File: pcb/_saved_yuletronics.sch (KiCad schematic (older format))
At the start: 52 parts, among them IC1 STM32F042F6P6, IC3 TLV61225, J1 BATT, J2 MICROUSB, J3 CONN_01x08, P1 SWD_TC, SW1 BOOTLOAD, SW2 PWR_SWITCH, SW3 BOOTLOAD, U1 XC6210B332MR, U2 ULN2003D1013TR, X1 Silk_art

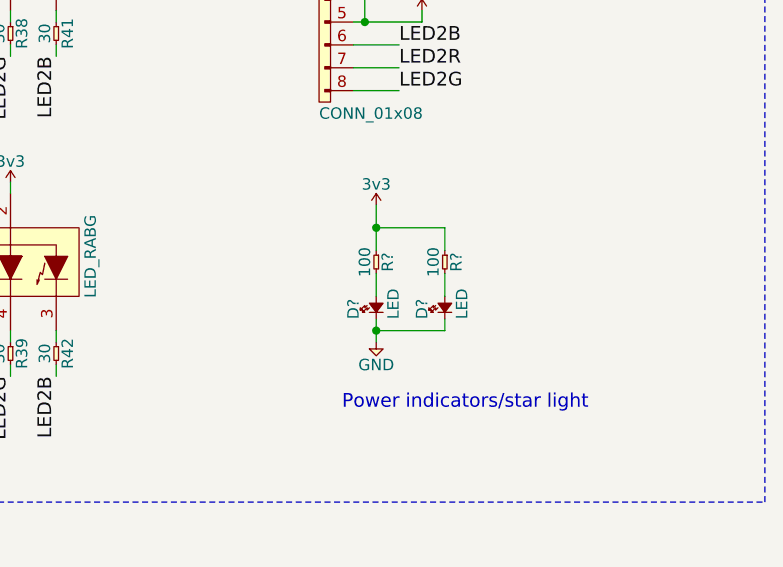
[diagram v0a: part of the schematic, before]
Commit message: Fix circuit to account for LED currents: change resistor values, upgrade LDO regulator, use transistor array
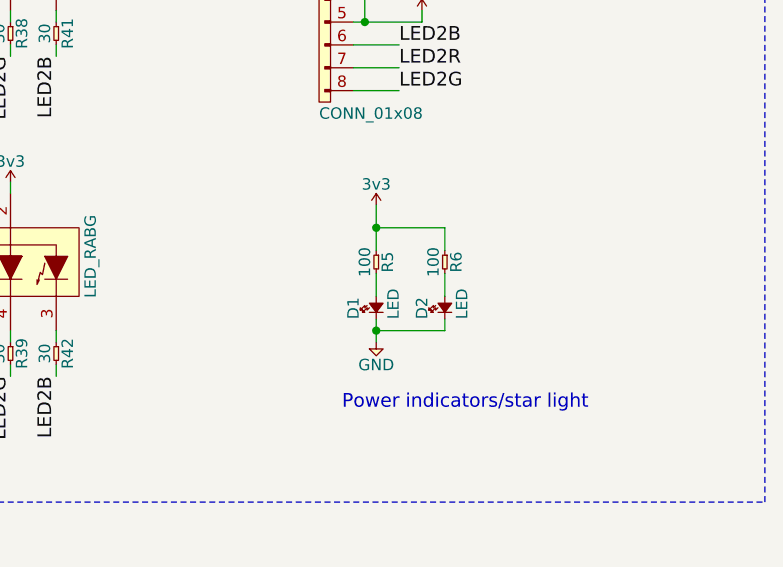
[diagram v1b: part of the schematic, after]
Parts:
- gave numbers to parts that had none: 4
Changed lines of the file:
@@
 	4250 5350 4250 5200
 $Comp
-L LED D?
+L LED D1
 U 1 1 58097B31
 P 9200 4700
-F 0 "D?" H 9200 4800 50  0000 L CNN
+F 0 "D1" H 9200 4800 50  0000 L CNN
 F 1 "LED" H 9200 4625 50  0000 L CNN
 F 2 "agg:0805-LED" H 9200 4700 50  0001 C CNN
@@
 $EndComp
 $Comp
-L 3v3 #PWR?
+L 3v3 #PWR038
 U 1 1 58098160
 P 9200 4200
-F 0 "#PWR?" H 9200 4310 50  0001 L CNN
+F 0 "#PWR038" H 9200 4310 50  0001 L CNN
 F 1 "3v3" H 9200 4290 50  0000 C CNN
 F 2 "" H 9200 4200 60  0001 C CNN
@@
 $EndComp
 $Comp
-L GND #PWR?
+L GND #PWR039
 U 1 1 580987D6
 P 9200 4800
-F 0 "#PWR?" H 9070 4840 50  0001 L CNN
+F 0 "#PWR039" H 9070 4840 50  0001 L CNN
 F 1 "GND" H 9200 4700 50  0000 C CNN
 F 2 "" H 9200 4800 60  0001 C CNN
@@
 Power indicators/star light
 $Comp
-L LED D?
+L LED D2
 U 1 1 580998C3
 P 9500 4700
-F 0 "D?" H 9500 4800 50  0000 L CNN
+F 0 "D2" H 9500 4800 50  0000 L CNN
 F 1 "LED" H 9500 4625 50  0000 L CNN
 F 2 "agg:0805-LED" H 9500 4700 50  0001 C CNN
@@
 $EndComp
 $Comp
-L R R?
+L R R5
 U 1 1 58099A5B
 P 9200 4400
-F 0 "R?" H 9250 4450 50  0000 C CNN
+F 0 "R5" H 9250 4450 50  0000 C CNN
 F 1 "100" H 9250 4350 50  0000 C CNN
 F 2 "agg:0805" H 9200 4400 50  0001 C CNN
@@
 $EndComp
 $Comp
-L R R?
+L R R6
 U 1 1 58099CFF
 P 9500 4400
-F 0 "R?" H 9550 4450 50  0000 C CNN
+F 0 "R6" H 9550 4450 50  0000 C CNN
 F 1 "100" H 9550 4350 50  0000 C CNN
 F 2 "agg:0805" H 9500 4400 50  0001 C CNN

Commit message: Further configuration, create initial board.h file
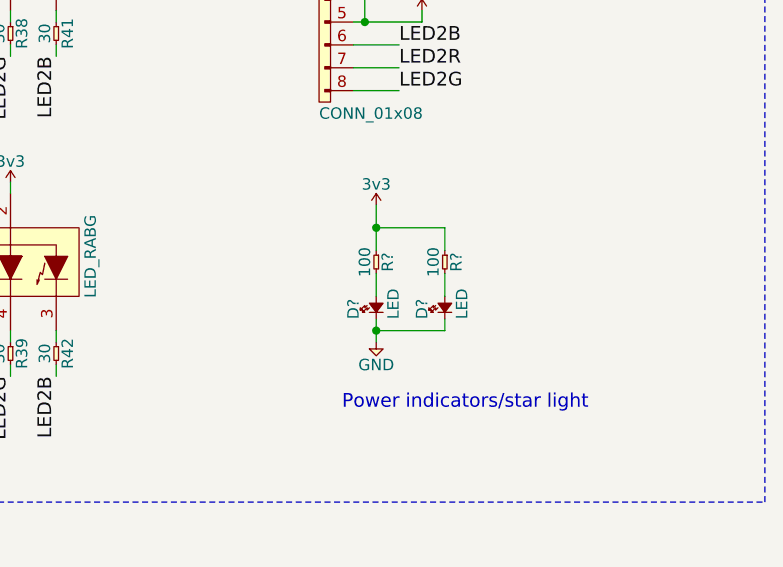
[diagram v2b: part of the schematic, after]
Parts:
- renumbered D1 to D?, D2 to D?, R5 to R?, R6 to R?
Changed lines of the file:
@@
 	4250 5350 4250 5200
 $Comp
-L LED D1
+L LED D?
 U 1 1 58097B31
 P 9200 4700
-F 0 "D1" H 9200 4800 50  0000 L CNN
+F 0 "D?" H 9200 4800 50  0000 L CNN
 F 1 "LED" H 9200 4625 50  0000 L CNN
 F 2 "agg:0805-LED" H 9200 4700 50  0001 C CNN
@@
 $EndComp
 $Comp
-L 3v3 #PWR038
+L 3v3 #PWR?
 U 1 1 58098160
 P 9200 4200
-F 0 "#PWR038" H 9200 4310 50  0001 L CNN
+F 0 "#PWR?" H 9200 4310 50  0001 L CNN
 F 1 "3v3" H 9200 4290 50  0000 C CNN
 F 2 "" H 9200 4200 60  0001 C CNN
@@
 $EndComp
 $Comp
-L GND #PWR039
+L GND #PWR?
 U 1 1 580987D6
 P 9200 4800
-F 0 "#PWR039" H 9070 4840 50  0001 L CNN
+F 0 "#PWR?" H 9070 4840 50  0001 L CNN
 F 1 "GND" H 9200 4700 50  0000 C CNN
 F 2 "" H 9200 4800 60  0001 C CNN
@@
 Power indicators/star light
 $Comp
-L LED D2
+L LED D?
 U 1 1 580998C3
 P 9500 4700
-F 0 "D2" H 9500 4800 50  0000 L CNN
+F 0 "D?" H 9500 4800 50  0000 L CNN
 F 1 "LED" H 9500 4625 50  0000 L CNN
 F 2 "agg:0805-LED" H 9500 4700 50  0001 C CNN
@@
 $EndComp
 $Comp
-L R R5
+L R R?
 U 1 1 58099A5B
 P 9200 4400
-F 0 "R5" H 9250 4450 50  0000 C CNN
+F 0 "R?" H 9250 4450 50  0000 C CNN
 F 1 "100" H 9250 4350 50  0000 C CNN
 F 2 "agg:0805" H 9200 4400 50  0001 C CNN
@@
 $EndComp
 $Comp
-L R R6
+L R R?
 U 1 1 58099CFF
 P 9500 4400
-F 0 "R6" H 9550 4450 50  0000 C CNN
+F 0 "R?" H 9550 4450 50  0000 C CNN
 F 1 "100" H 9550 4350 50  0000 C CNN
 F 2 "agg:0805" H 9500 4400 50  0001 C CNN
